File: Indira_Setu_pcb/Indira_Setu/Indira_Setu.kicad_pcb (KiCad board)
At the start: 2 copper layers, 144.5 x 55 mm, 2 parts, among them U1 Pico

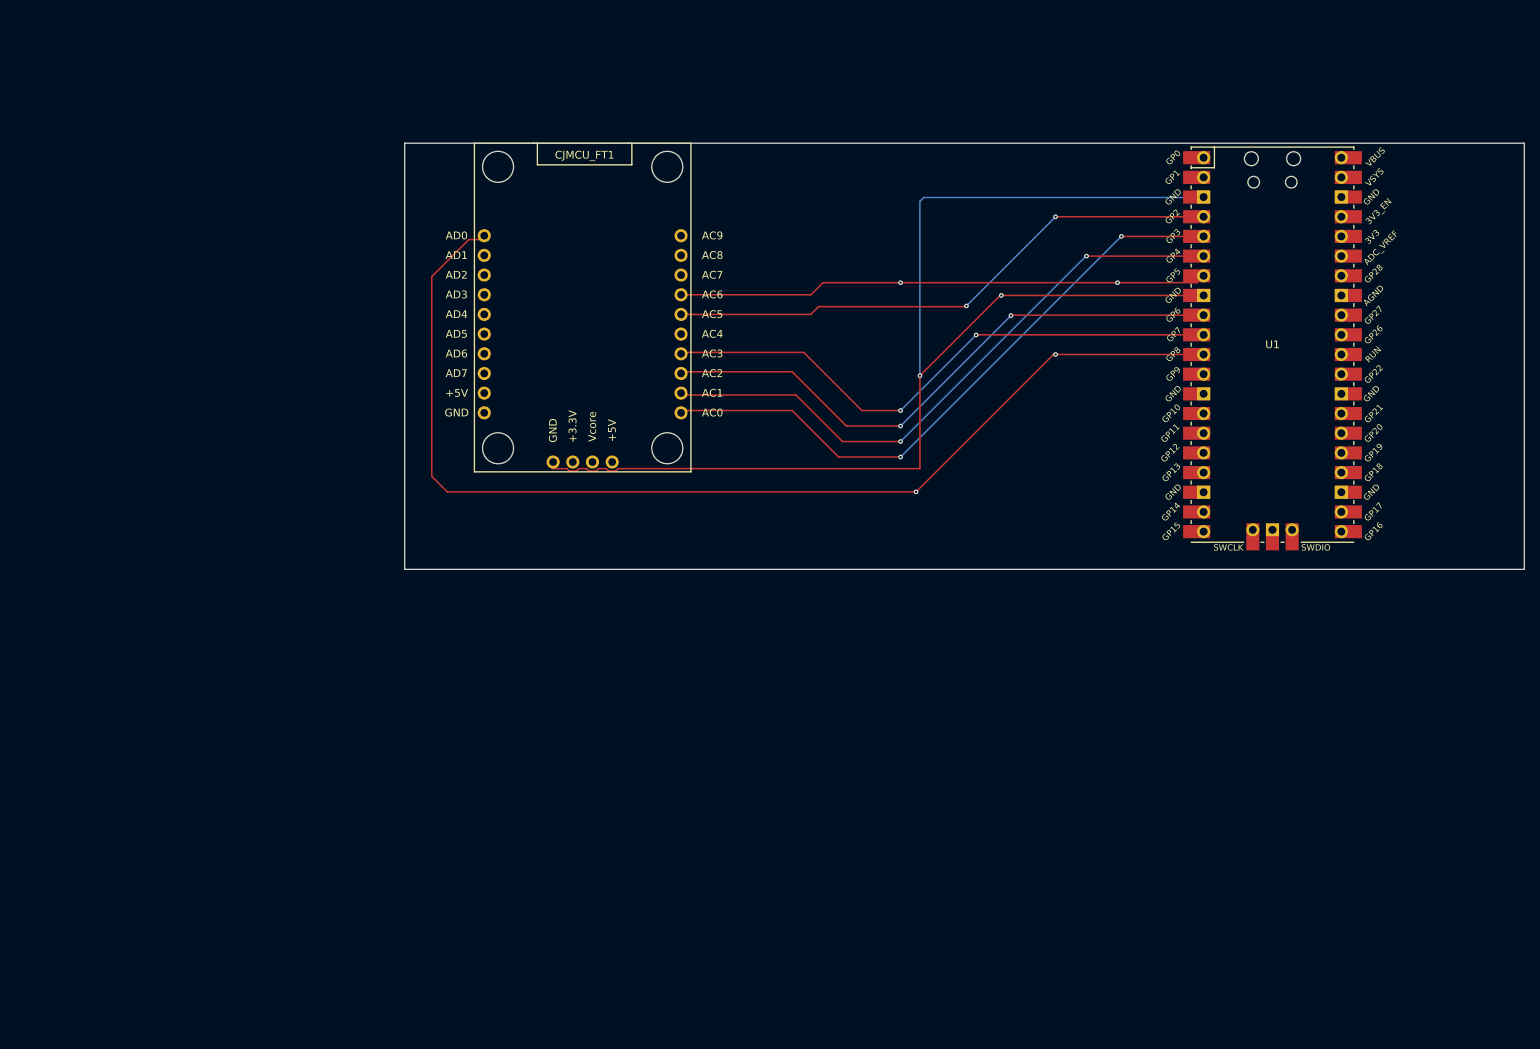
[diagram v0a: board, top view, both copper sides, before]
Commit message: Add files via upload
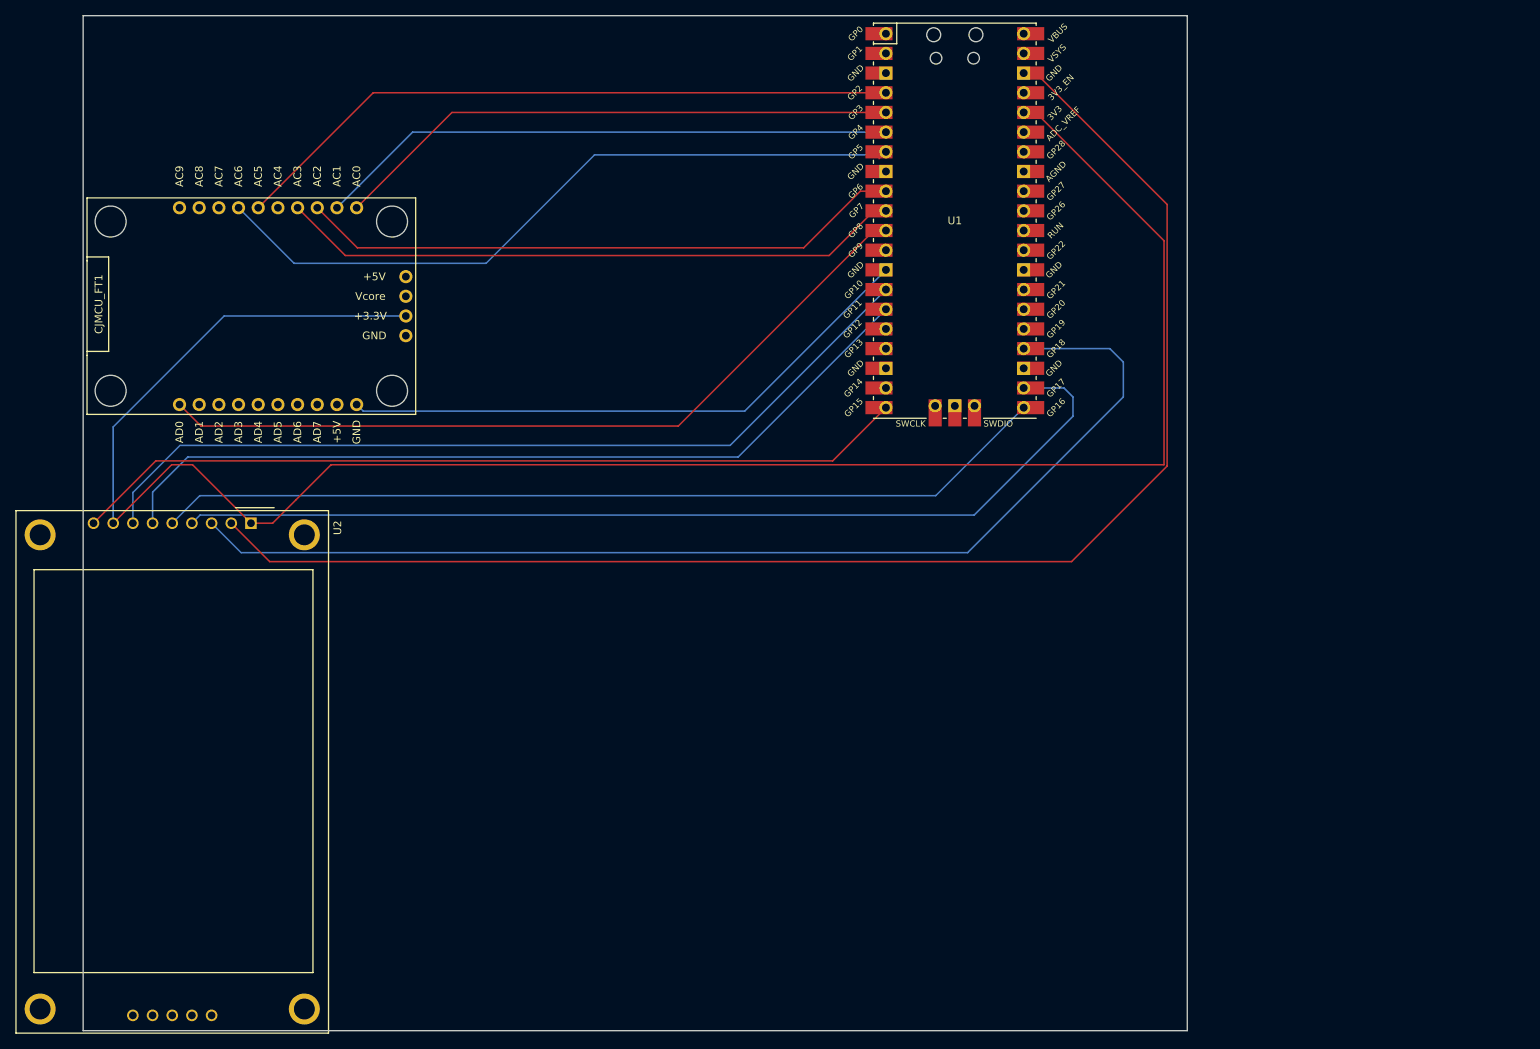
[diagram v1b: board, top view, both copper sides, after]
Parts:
- added U2: CR2013-MI2120, Display:CR2013-MI2120, F.Cu at (75.7, 95.5)
- moved CJMCU_FT1 61.0 mm to (54.5, 81.5), turned to 90 degrees
- moved U1 44.0 mm to (166.5, 56.5)
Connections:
- CJMCU_FT1 pad +3.3V: unconnected-(CJMCU_FT1-Pad+3.3V) -> Net-(U1-3V3)
- CJMCU_FT1 pad GND1: unconnected-(CJMCU_FT1-GND-PadGND1) -> Net-(CJMCU_FT1-GND-PadGND1)
- CJMCU_FT1 pad GND2: Net-(CJMCU_FT1-GND-PadGND2) -> unconnected-(CJMCU_FT1-GND-PadGND2)
- U1 pad 13: unconnected-(U1-GND-Pad13) -> Net-(CJMCU_FT1-GND-PadGND1)
- U1 pad 14: unconnected-(U1-GPIO10-Pad14) -> Net-(U1-GPIO10)
- U1 pad 15: unconnected-(U1-GPIO11-Pad15) -> Net-(U1-GPIO11)
- U1 pad 20: unconnected-(U1-GPIO15-Pad20) -> Net-(U1-GPIO15)
- U1 pad 21: unconnected-(U1-GPIO16-Pad21) -> Net-(U1-GPIO16)
- U1 pad 22: unconnected-(U1-GPIO17-Pad22) -> Net-(U1-GPIO17)
- U1 pad 24: unconnected-(U1-GPIO18-Pad24) -> Net-(U1-GPIO18)
- U1 pad 3: Net-(CJMCU_FT1-GND-PadGND2) -> unconnected-(U1-GND-Pad3)
- U1 pad 36: unconnected-(U1-3V3-Pad36) -> Net-(U1-3V3)
- U1 pad 38: unconnected-(U1-GND-Pad38) -> Net-(U2-GND)
- U1 pad 8: Net-(CJMCU_FT1-GND-PadGND2) -> unconnected-(U1-GND-Pad8)
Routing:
- net Net-(U1-3V3): track 0.00 -> 255.0 mm
- net Net-(U2-GND): track 0.00 -> 187.2 mm
- net Net-(CJMCU_FT1-GND-PadGND2): track 161.4 -> 0.00 mm, vias 2 -> 0
- net Net-(U1-GPIO18): track 0.00 -> 145.6 mm
- net Net-(U1-GPIO17): track 0.00 -> 128.8 mm
- net Net-(U1-GPIO16): track 0.00 -> 116.1 mm
- net Net-(U1-GPIO10): track 0.00 -> 112.0 mm
- net Net-(U1-GPIO15): track 0.00 -> 108.4 mm
- net Net-(U1-GPIO11): track 0.00 -> 108.4 mm
- net Net-(CJMCU_FT1-GND-PadGND1): track 0.00 -> 76.2 mm
- net Net-(U1-GPIO8): track 142.5 -> 102.8 mm, vias 2 -> 0
- net Net-(U1-GPIO5): track 68.5 -> 93.0 mm, vias 2 -> 0
- net Net-(U1-GPIO2): track 72.7 -> 87.2 mm, vias 2 -> 0
- net Net-(U1-GPIO3): track 81.8 -> 73.4 mm, vias 2 -> 0
- net Net-(U1-GPIO7): track 74.7 -> 80.9 mm, vias 2 -> 0
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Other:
- board size 144.5 x 55 mm -> 142.5 x 131 mm
